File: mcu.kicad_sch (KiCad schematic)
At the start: 14 parts, among them SW1 SW_Push, U1 ATmega328P-A, Y1 16Mhz

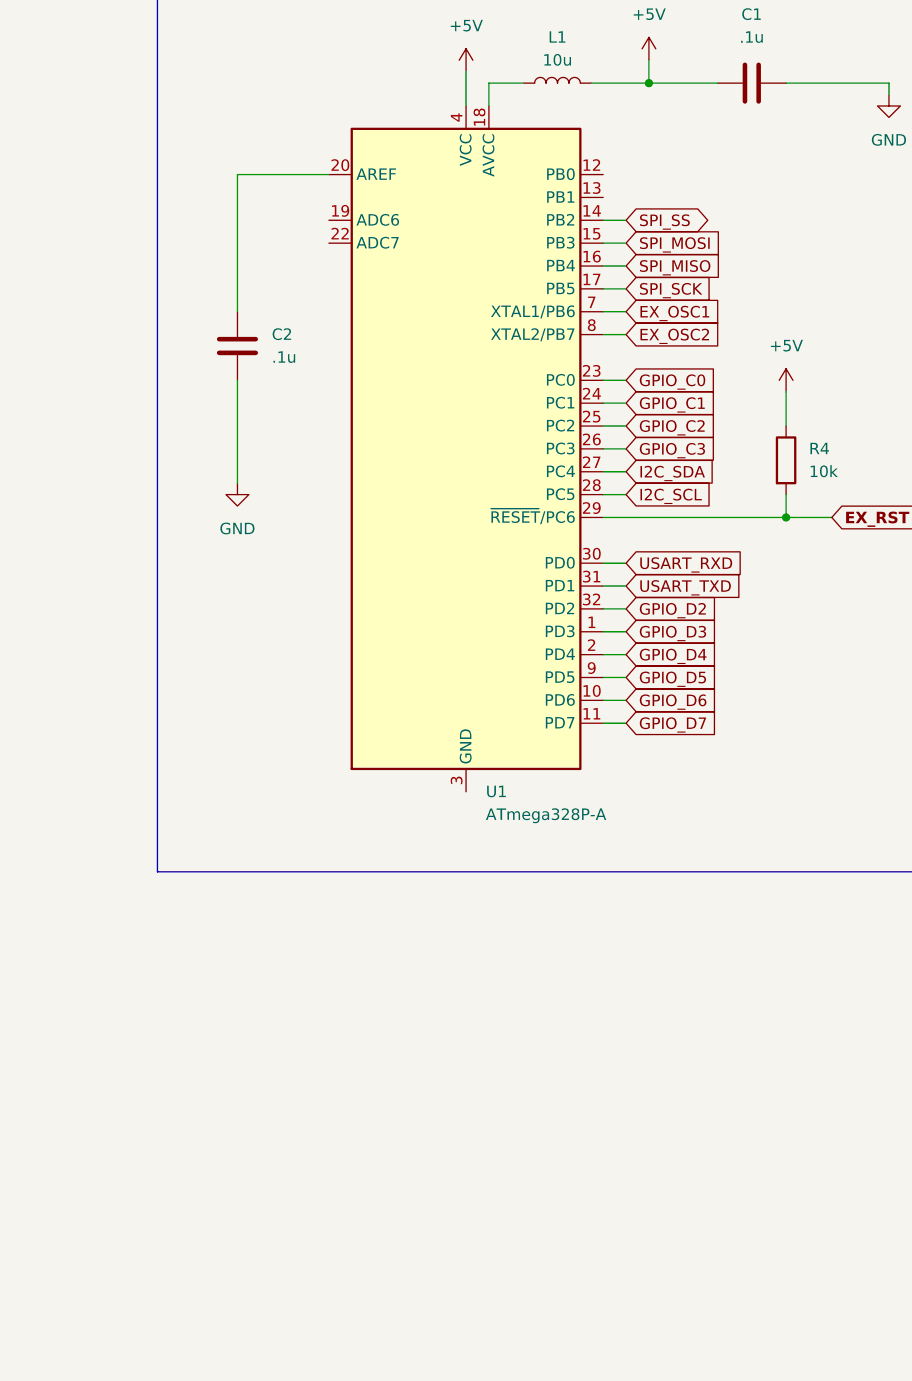
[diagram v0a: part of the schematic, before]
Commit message: Fixing git
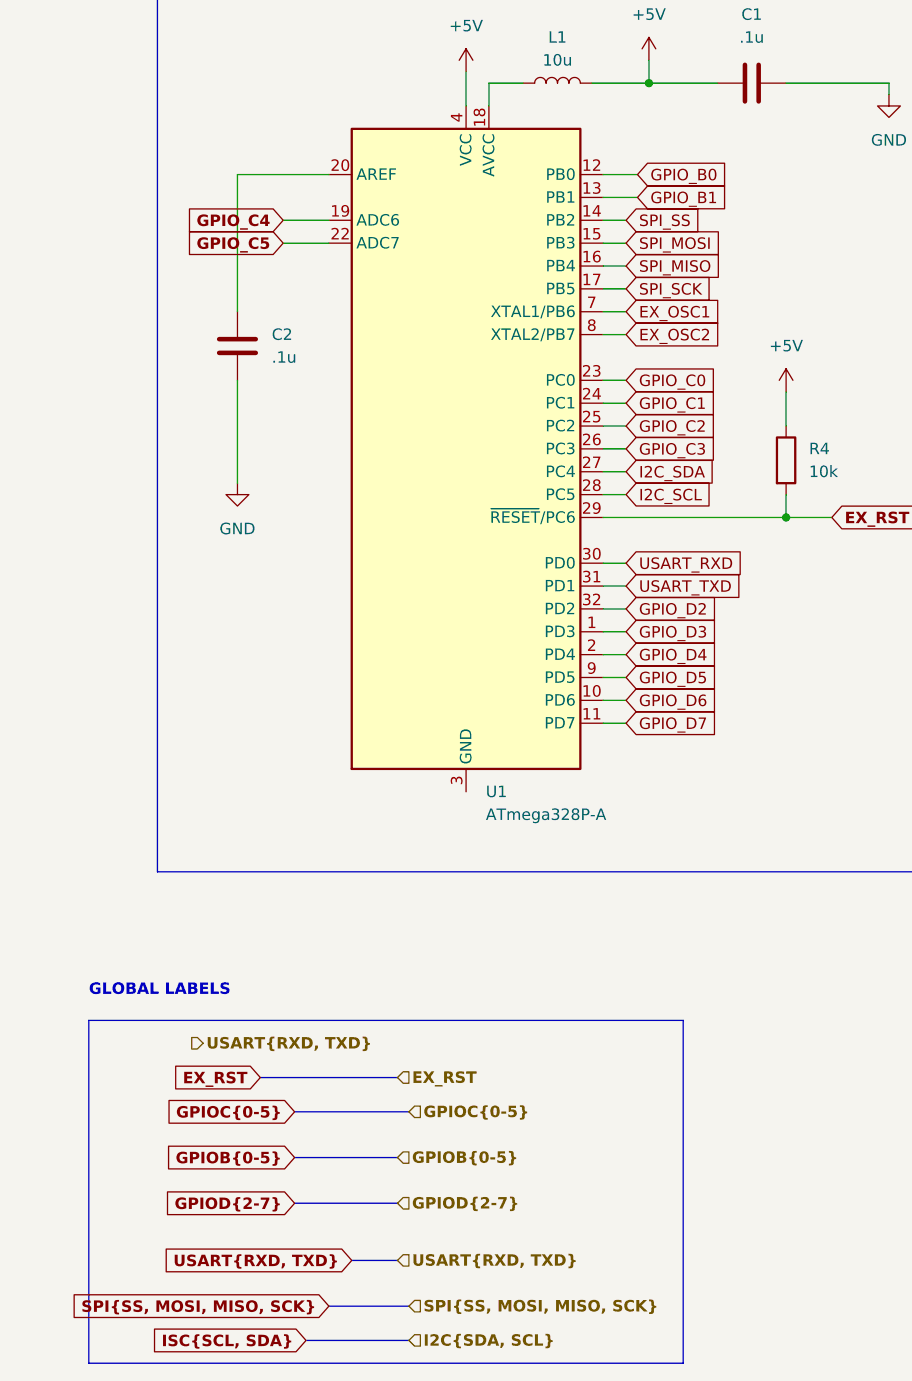
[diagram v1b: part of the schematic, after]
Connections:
- net GPIO_B0: now reaches U1.12 (PB0)
- net GPIO_B1: now reaches U1.13 (PB1)
- net GPIO_C4: now reaches U1.19 (ADC6)
- net GPIO_C5: now reaches U1.22 (ADC7)
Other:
- note added: "GLOBAL LABELS"
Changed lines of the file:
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@@
+    (stroke (width 0) (type default))
+  )
+  (bus (pts (xy 49.53 167.64) (xy 60.96 167.64))
     (stroke (width 0) (type default))
   )
@@
     (stroke (width 0) (type default))
   )
+  (wire (pts (xy 83.82 53.34) (xy 87.63 53.34))
+    (stroke (width 0) (type default))
+  )
   (wire (pts (xy 83.82 101.6) (xy 86.36 101.6))
     (stroke (width 0) (type default))
@@
     (stroke (width 0) (type default))
   )
+  (bus (pts (xy 50.8 182.88) (xy 62.23 182.88))
+    (stroke (width 0) (type default))
+  )
   (wire (pts (xy 83.82 114.3) (xy 86.36 114.3))
     (stroke (width 0) (type default))
@@
     (stroke (width 0) (type default))
   )
+  (wire (pts (xy 48.26 60.96) (xy 53.34 60.96))
+    (stroke (width 0) (type default))
+  )
+  (wire (pts (xy 48.26 58.42) (xy 53.34 58.42))
+    (stroke (width 0) (type default))
+  )
   (wire (pts (xy 104.14 77.47) (xy 104.14 81.28))
     (stroke (width 0) (type default))
@@
     (stroke (width 0) (type default))
   )
+  (bus (pts (xy 53.34 179.07) (xy 62.23 179.07))
+    (stroke (width 0) (type default))
+  )
   (wire (pts (xy 83.82 83.82) (xy 86.36 83.82))
     (stroke (width 0) (type default))
@@
     (stroke (width 0) (type default))
   )
+  (bus (pts (xy 55.88 173.99) (xy 60.96 173.99))
+    (stroke (width 0) (type default))
+  )
   (wire (pts (xy 83.82 91.44) (xy 104.14 91.44))
     (stroke (width 0) (type default))
@@
     (stroke (width 0) (type default))
   )
+  (bus (pts (xy 45.72 153.67) (xy 60.96 153.67))
+    (stroke (width 0) (type default))
+  )
+  (bus (pts (xy 49.53 157.48) (xy 62.23 157.48))
+    (stroke (width 0) (type default))
+  )
   (wire (pts (xy 238.76 134.62) (xy 250.19 134.62))
     (stroke (width 0) (type default))
@@
     (stroke (width 0) (type default))
   )
+  (bus (pts (xy 49.53 162.56) (xy 60.96 162.56))
+    (stroke (width 0) (type default))
+  )
   (wire (pts (xy 83.82 111.76) (xy 86.36 111.76))
+    (stroke (width 0) (type default))
+  )
+  (wire (pts (xy 83.82 55.88) (xy 87.63 55.88))
     (stroke (width 0) (type default))
   )
@@
     (fill (type none))
   )
+  (rectangle (start 26.67 147.32) (end 92.71 185.42)
+    (stroke (width 0) (type default))
+    (fill (type none))
+  )
   (rectangle (start 34.29 26.67) (end 120.65 130.81)
     (stroke (width 0) (type default))
@@
     (effects (font (size 1.27 1.27) (thickness 0.254) bold) (justify left bottom))
   )
+  (text "GLOBAL LABELS\n" (at 26.67 144.78 0)
+    (effects (font (size 1.27 1.27) bold) (justify left bottom))
+  )
   (global_label "EX_RST" (shape output) (at 152.4 119.38 0) (fields_autoplaced)
     (effects (font (size 1.27 1.27)) (justify left))
@@
     )
   )
+  (global_label "GPIOC{0-5}" (shape input) (at 49.53 157.48 180) (fields_autoplaced)
+    (effects (font (size 1.27 1.27) bold) (justify right))
+    (property "Intersheetrefs" "${INTERSHEET_REFS}" (at 34.6387 157.48 0)
+      (effects (font (size 1.27 1.27)) (justify right) hide)
+    )
+  )
   (global_label "USART_TXD" (shape input) (at 86.36 99.06 0) (fields_autoplaced)
     (effects (font (size 1.27 1.27)) (justify left))
@@
     )
   )
+  (global_label "GPIO_C5" (shape input) (at 48.26 60.96 180) (fields_autoplaced)
+    (effects (font (size 1.27 1.27) bold) (justify right))
+    (property "Intersheetrefs" "${INTERSHEET_REFS}" (at 36.8764 60.96 0)
+      (effects (font (size 1.27 1.27)) (justify right) hide)
+    )
+  )
   (global_label "I2C_SCL" (shape output) (at 218.44 91.44 0) (fields_autoplaced)
     (effects (font (size 1.27 1.27)) (justify left))
@@
     )
   )
+  (global_label "GPIO_B0" (shape input) (at 87.63 53.34 0) (fields_autoplaced)
+    (effects (font (size 1.27 1.27)) (justify left))
+    (property "Intersheetrefs" "${INTERSHEET_REFS}" (at 98.5376 53.34 0)
+      (effects (font (size 1.27 1.27)) (justify left) hide)
+    )
+  )
   (global_label "GPIO_D4" (shape input) (at 86.36 106.68 0) (fields_autoplaced)
     (effects (font (size 1.27 1.27)) (justify left))
@@
     )
   )
+  (global_label "GPIOB{0-5}" (shape input) (at 49.53 162.56 180) (fields_autoplaced)
+    (effects (font (size 1.27 1.27) bold) (justify right))
+    (property "Intersheetrefs" "${INTERSHEET_REFS}" (at 34.6387 162.56 0)
+      (effects (font (size 1.27 1.27)) (justify right) hide)
+    )
+  )
   (global_label "USART_RXD" (shape input) (at 86.36 96.52 0) (fields_autoplaced)
     (effects (font (size 1.27 1.27)) (justify left))
@@
     )
   )
+  (global_label "GPIO_C4" (shape input) (at 48.26 58.42 180) (fields_autoplaced)
+    (effects (font (size 1.27 1.27) bold) (justify right))
+    (property "Intersheetrefs" "${INTERSHEET_REFS}" (at 36.8764 58.42 0)
+      (effects (font (size 1.27 1.27)) (justify right) hide)
+    )
+  )
+  (global_label "ISC{SCL, SDA}" (shape input) (at 50.8 182.88 180) (fields_autoplaced)
+    (effects (font (size 1.27 1.27) bold) (justify right))
+    (property "Intersheetrefs" "${INTERSHEET_REFS}" (at 33.913 182.88 0)
+      (effects (font (size 1.27 1.27)) (justify right) hide)
+    )
+  )
   (global_label "I2C_SDA" (shape output) (at 218.44 86.36 0) (fields_autoplaced)
     (effects (font (size 1.27 1.27)) (justify left))
@@
     )
   )
+  (global_label "SPI{SS, MOSI, MISO, SCK}" (shape input) (at 53.34 179.07 180) (fields_autoplaced)
+    (effects (font (size 1.27 1.27) bold) (justify right))
+    (property "Intersheetrefs" "${INTERSHEET_REFS}" (at 25.023 179.07 0)
+      (effects (font (size 1.27 1.27)) (justify right) hide)
+    )
+  )
   (global_label "GPIO_C1" (shape input) (at 86.36 78.74 0) (fields_autoplaced)
     (effects (font (size 1.27 1.27)) (justify left))
@@
     )
   )
+  (global_label "GPIO_B1" (shape input) (at 87.63 55.88 0) (fields_autoplaced)
+    (effects (font (size 1.27 1.27)) (justify left))
+    (property "Intersheetrefs" "${INTERSHEET_REFS}" (at 98.5376 55.88 0)
+      (effects (font (size 1.27 1.27)) (justify left) hide)
+    )
+  )
   (global_label "EX_OSC2" (shape output) (at 220.98 134.62 0) (fields_autoplaced)
     (effects (font (size 1.27 1.27)) (justify left))
@@
     )
   )
+  (global_label "USART{RXD, TXD}" (shape input) (at 55.88 173.99 180) (fields_autoplaced)
+    (effects (font (size 1.27 1.27) bold) (justify right))
+    (property "Intersheetrefs" "${INTERSHEET_REFS}" (at 36.0902 173.99 0)
+      (effects (font (size 1.27 1.27)) (justify right) hide)
+    )
+  )
   (global_label "GPIO_C3" (shape input) (at 86.36 83.82 0) (fields_autoplaced)
     (effects (font (size 1.27 1.27)) (justify left))
@@
     )
   )
+  (global_label "GPIOD{2-7}" (shape input) (at 49.53 167.64 180) (fields_autoplaced)
+    (effects (font (size 1.27 1.27) bold) (justify right))
+    (property "Intersheetrefs" "${INTERSHEET_REFS}" (at 34.6387 167.64 0)
+      (effects (font (size 1.27 1.27)) (justify right) hide)
+    )
+  )
   (global_label "GPIO_D6" (shape input) (at 86.36 111.76 0) (fields_autoplaced)
     (effects (font (size 1.27 1.27)) (justify left))
@@
     )
   )
+  (global_label "EX_RST" (shape input) (at 45.72 153.67 180) (fields_autoplaced)
+    (effects (font (size 1.27 1.27) bold) (justify right))
+    (property "Intersheetrefs" "${INTERSHEET_REFS}" (at 35.4856 153.67 0)
+      (effects (font (size 1.27 1.27)) (justify right) hide)
+    )
+  )
   (global_label "EX_RST" (shape input) (at 109.22 91.44 0) (fields_autoplaced)
     (effects (font (size 1.27 1.27) bold) (justify left))
@@
     )
   )
-  (global_label "SPI_SS" (shape bidirectional) (at 86.36 58.42 0) (fields_autoplaced)
-    (effects (font (size 1.27 1.27)) (justify left))
-    (property "Intersheetrefs" "${INTERSHEET_REFS}" (at 96.9274 58.42 0)
+  (global_label "SPI_SS" (shape input) (at 86.36 58.42 0) (fields_autoplaced)
+    (effects (font (size 1.27 1.27)) (justify left))
+    (property "Intersheetrefs" "${INTERSHEET_REFS}" (at 95.8161 58.42 0)
       (effects (font (size 1.27 1.27)) (justify left) hide)
     )
@@
     )
   )
+  (hierarchical_label "GPIOD{2-7}" (shape input) (at 60.96 167.64 0) (fields_autoplaced)
+    (effects (font (size 1.27 1.27) bold) (justify left))
+  )
+  (hierarchical_label "GPIOC{0-5}" (shape input) (at 62.23 157.48 0) (fields_autoplaced)
+    (effects (font (size 1.27 1.27) bold) (justify left))
+  )
+  (hierarchical_label "USART{RXD, TXD}" (shape input) (at 60.96 173.99 0) (fields_autoplaced)
+    (effects (font (size 1.27 1.27) bold) (justify left))
+  )
+  (hierarchical_label "I2C{SDA, SCL}" (shape input) (at 62.23 182.88 0) (fields_autoplaced)
+    (effects (font (size 1.27 1.27) bold) (justify left))
+  )
+  (hierarchical_label "USART{RXD, TXD}" (shape output) (at 38.1 149.86 0) (fields_autoplaced)
+    (effects (font (size 1.27 1.27) bold) (justify left))
+  )
+  (hierarchical_label "SPI{SS, MOSI, MISO, SCK}" (shape input) (at 62.23 179.07 0) (fields_autoplaced)
+    (effects (font (size 1.27 1.27) bold) (justify left))
+  )
+  (hierarchical_label "EX_RST" (shape input) (at 60.96 153.67 0) (fields_autoplaced)
+    (effects (font (size 1.27 1.27) bold) (justify left))
+  )
+  (hierarchical_label "GPIOB{0-5}" (shape input) (at 60.96 162.56 0) (fields_autoplaced)
+    (effects (font (size 1.27 1.27) bold) (justify left))
+  )
   (symbol (lib_id "Device:C") (at 265.43 134.62 90) (unit 1)
